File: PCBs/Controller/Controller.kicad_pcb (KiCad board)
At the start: 2 copper layers, 100 x 62.4 mm, 62 parts, among them J1 USB_B_Micro, J2 Micro_SD_Card_Det1, J3 RS485, J4 UART, J5 TagConnect, Q1 PMOS, SW1 NSRT Swtich, SW2 NSRT Swtich, U1 STM32F030R8Tx, U2 TPS62125DSG, U3 Salinity, U4 Depth, U5 ERD210RS, U6 ERD210RS, U7 ERD210RS, U8 SP3485EN

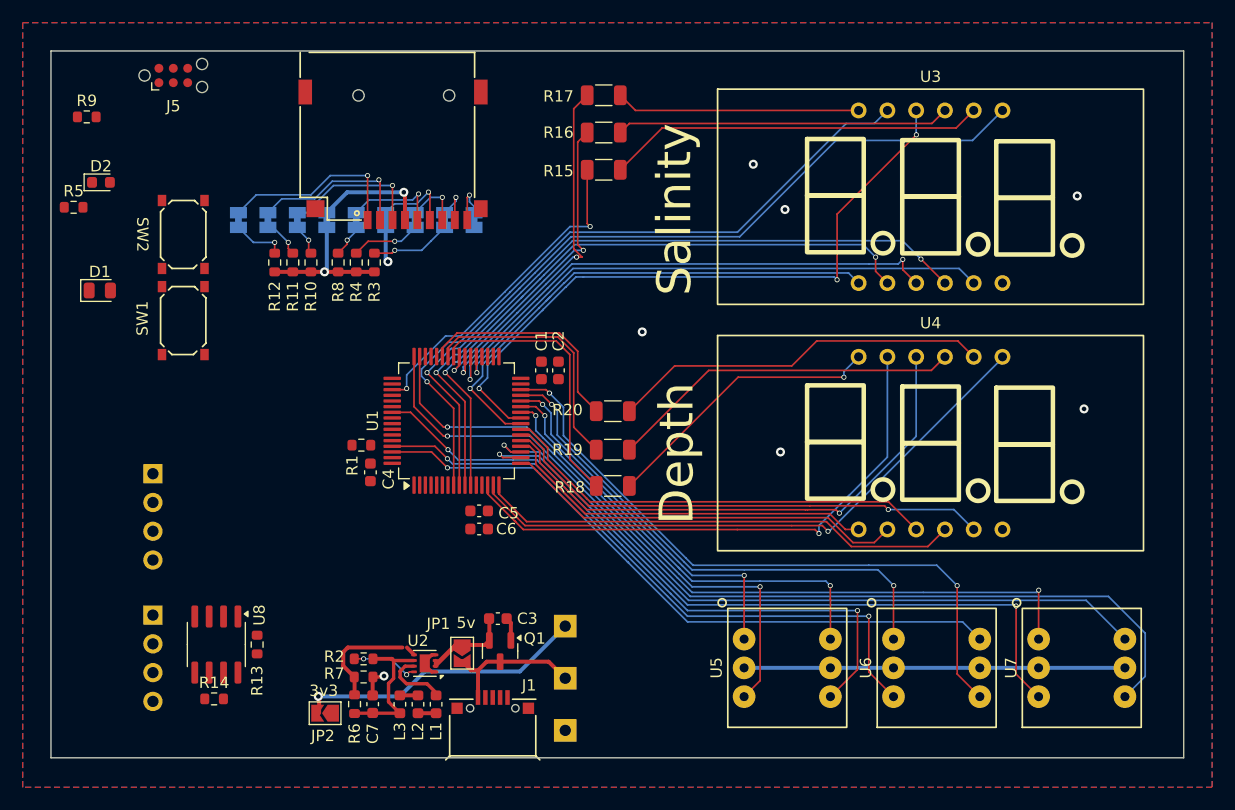
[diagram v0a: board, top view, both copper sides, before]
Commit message: kicad changes
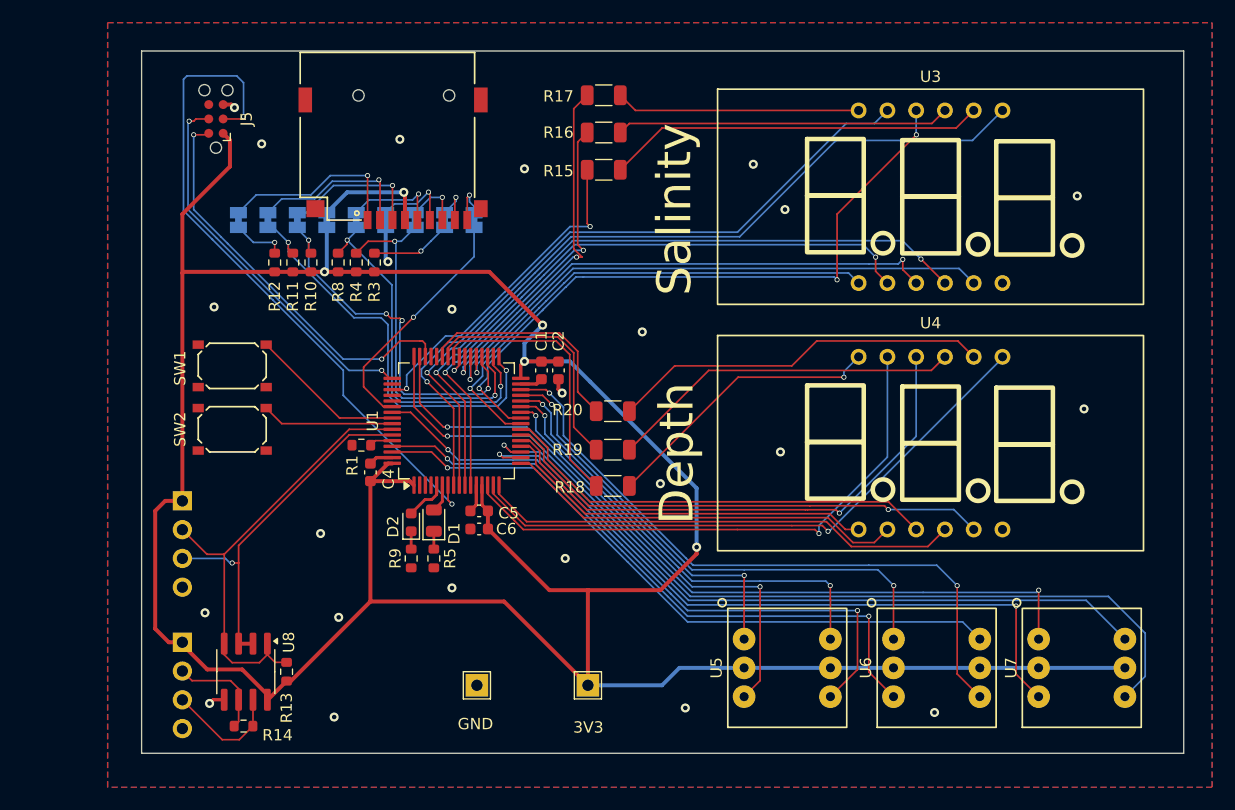
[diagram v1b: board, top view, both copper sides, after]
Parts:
- removed C3, C7: 10u, Capacitor_SMD:C_0603_1608Metric
- removed J1: USB_B_Micro, 4022S:microUSB
- removed JP1: ReversePolarity, Jumper:SolderJumper-2_P1.3mm_Open_TrianglePad1.0x1.5mm
- removed JP2: SolderJumper_2_Open, Jumper:SolderJumper-2_P1.3mm_Open_TrianglePad1.0x1.5mm
- removed L1, L2, L3: 4.7u, Inductor_SMD:L_0603_1608Metric
- removed Q1: PMOS, Package_TO_SOT_SMD:SOT-23
- removed R2: 100k, Resistor_SMD:R_0603_1608Metric
- removed R6: 4.7M, Resistor_SMD:R_0603_1608Metric
- removed R7: 1.5M, Resistor_SMD:R_0603_1608Metric
- removed TP1: 5V, TestPoint:TestPoint_THTPad_2.0x2.0mm_Drill1.0mm
- removed U2: TPS62125DSG, Package_SON:WSON-8-1EP_2x2mm_P0.5mm_EP0.9x1.6mm
- SW1, SW2: value NSRT Swtich -> Switch
- TP2, TP3: moved to F.Cu
- moved R9 48.4 mm to (181.8, 94.8), turned to -90 degrees
- moved R5 44.4 mm to (183.8, 94.8), turned to -90 degrees
- moved D2 40.6 mm to (181.8, 91.6), turned to 90 degrees
- moved D1 35.8 mm to (183.8, 91.5), turned to 90 degrees
- moved SW2 17.7 mm to (166.0, 83.4), turned to 180 degrees
- moved TP3 8.76 mm to (187.6, 106.0), turned to 0 degrees
- moved SW1 5.89 mm to (166.0, 77.8), turned to 180 degrees
- moved TP2 5.59 mm to (197.4, 106.0), turned to 0 degrees
- moved J5 5.37 mm to (164.6, 56.0), turned to 90 degrees
- moved R13 3.54 mm to (170.8, 104.8)
- moved J3 3.54 mm to (161.6, 102.2)
- moved J4 3.54 mm to (161.6, 89.7)
- moved R14 3.54 mm to (167.0, 109.6)
- moved U8 3.54 mm to (167.2, 104.8)
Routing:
- net +3V3: track 72.3 -> 267.1 mm, vias 2 -> 4
- net /NRST: track 0.00 -> 59.7 mm, vias 0 -> 2
- net /RS485_uart: track 0.00 -> 40.2 mm
- net /SWDIO: track 0.00 -> 35.8 mm, vias 0 -> 2
- net /SWCLK: track 0.00 -> 33.8 mm, vias 0 -> 2
- net /SPI_NSS: track 3.46 -> 37.1 mm, vias 1 -> 2
- net /RS485_DE: track 0.00 -> 32.7 mm, vias 0 -> 1
- net /SPI_MOSI: track 2.77 -> 32.8 mm, vias 1 -> 4
- net /SPI_SCK: track 2.94 -> 32.1 mm, vias 1 -> 2
- net /SPI_MISO: track 6.14 -> 32.3 mm, vias 1 -> 2
- net /CD: track 0.00 -> 21.4 mm, vias 0 -> 1
- net /SW1: track 0.00 -> 13.8 mm
- net +5V: track 12.8 -> 0.00 mm
- net Net-(JP2-A): track 12.5 -> 0.00 mm
- net /SW2: track 0.00 -> 11.7 mm
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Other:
- board size 100 x 62.4 mm -> 92 x 62 mm
- board text added: "Author: Cameron Clark University of Cape Town Salinometer Controller Board v0 22/08/2024"
- board text removed: "3v3"
- board text removed: "5V"
- board text removed: "5v"
